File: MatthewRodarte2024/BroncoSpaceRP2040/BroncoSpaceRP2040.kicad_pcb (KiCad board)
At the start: 2 copper layers, 60 x 68 mm, 42 parts, among them J1 USB_B_Micro, J2 Conn_01x02, J3 Conn_01x18, J4 Conn_01x18, Q1 2N3906, U1 RP2040, U2 NCP1117-3.3_SOT223, U3 W25Q128JVS, U4 TMP461xxRUN, Y1 ABM8-272-T3

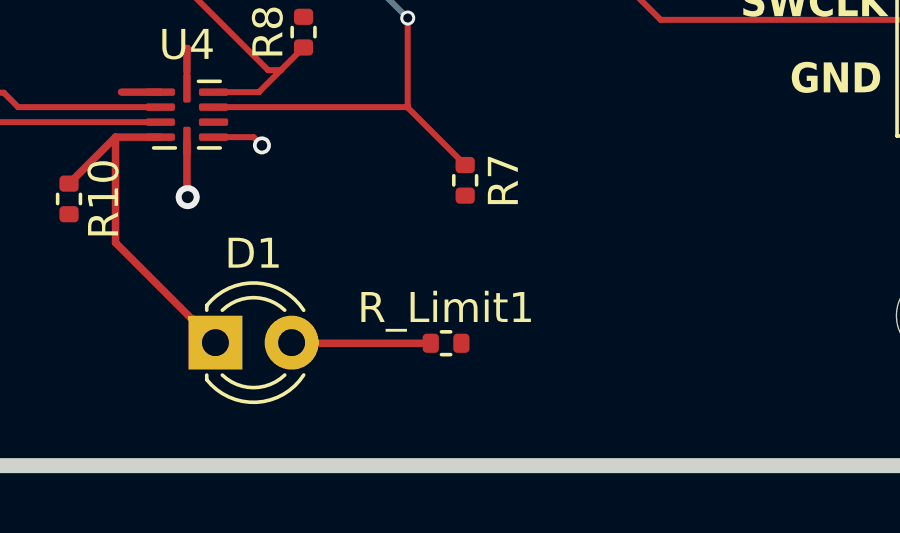
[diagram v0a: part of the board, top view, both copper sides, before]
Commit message: Updated stuff
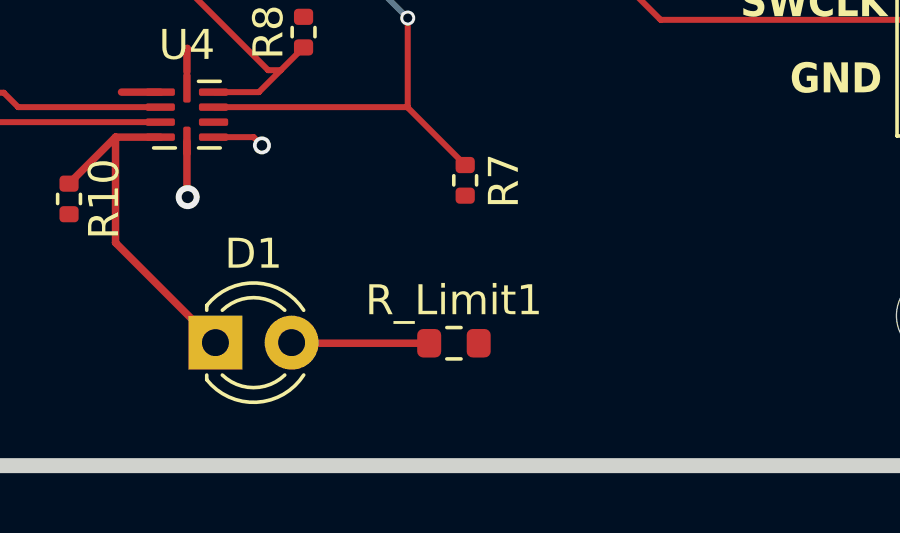
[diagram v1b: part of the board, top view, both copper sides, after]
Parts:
- R_Limit1: footprint Resistor_SMD:R_0402_1005Metric -> Resistor_SMD:R_0603_1608Metric
- moved R_Limit1 0.26 mm to (98.9, 123.9)
